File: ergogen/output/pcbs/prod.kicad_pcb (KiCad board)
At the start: 2 copper layers, 220.4 x 89.6 mm, 63 parts

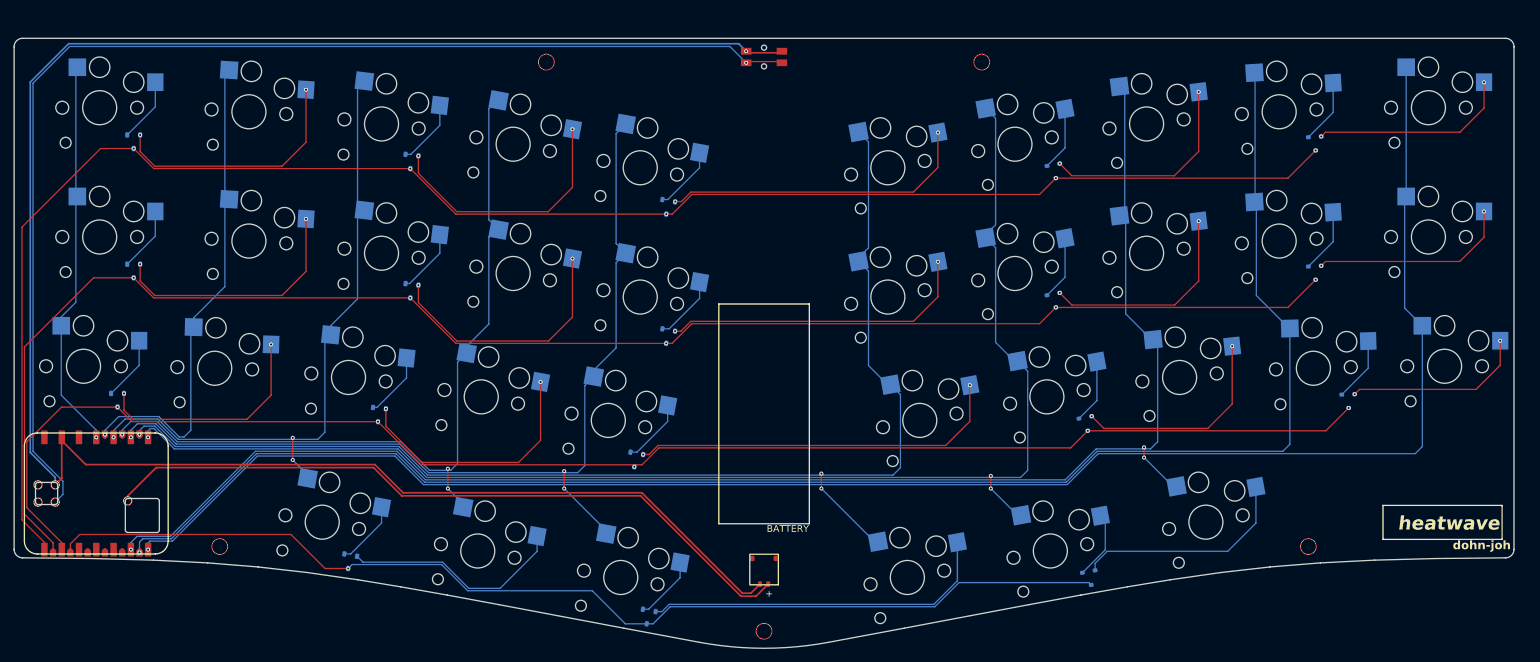
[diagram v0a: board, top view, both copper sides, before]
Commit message: release
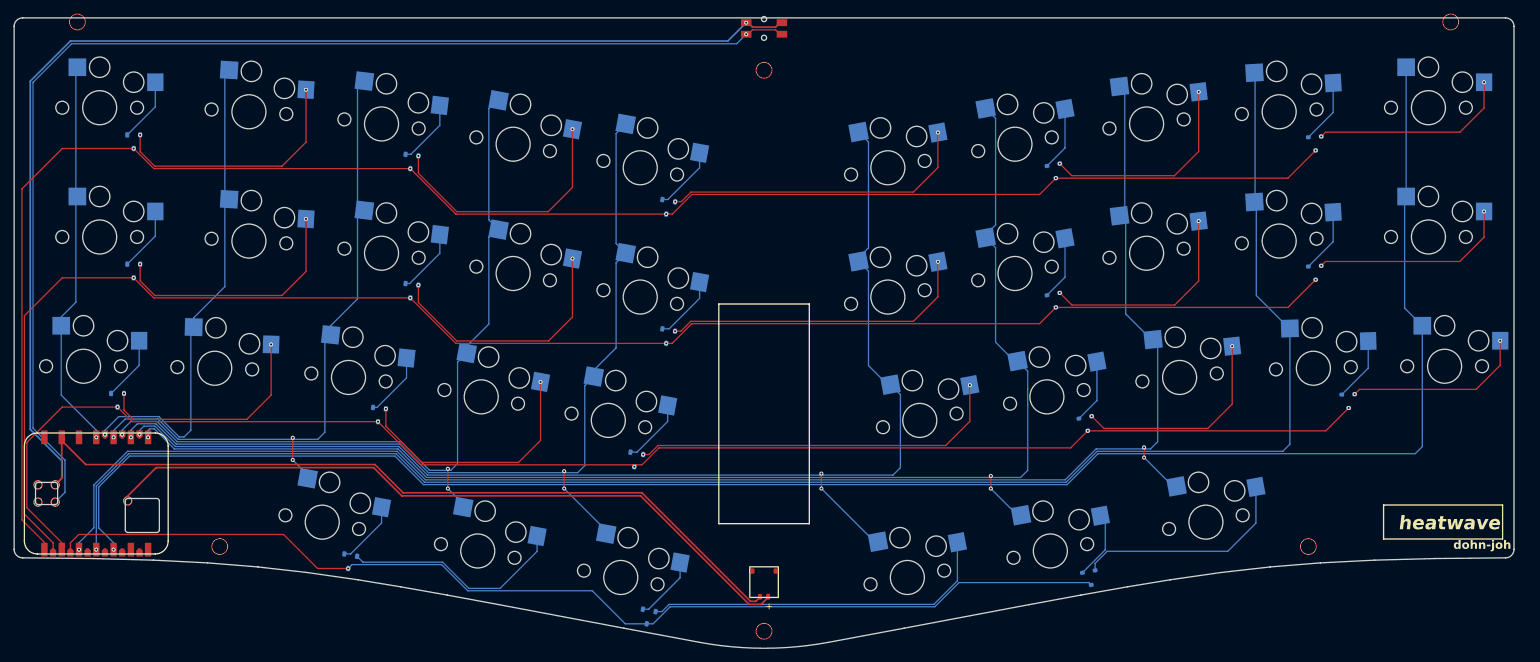
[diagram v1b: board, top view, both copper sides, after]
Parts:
- added H6: , mounting_hole, F.Cu at (177.6, 64.5)
- moved H3 196.7 mm to (198.6, -12.6)
- moved H4 81.0 mm to (17.6, 64.5)
- moved H5 81.0 mm to (97.6, 76.9)
- moved H1 69.2 mm to (-3.27, -12.6)
- moved H2 32.0 mm to (97.6, -5.50)
- moved XX1 4.20 mm to (97.6, -11.7)
- moved XX2 1.85 mm to (97.6, 70.0)
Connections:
- MCU1 pad 3: P0.28 -> C8
- MCU1 pad 4: P0.29 -> C9
- MCU1 pad 5: P0.04 -> C10
- MCU1 pad 6: C8 -> P0.05
- MCU1 pad 7: C10 -> P1.11
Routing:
- net C10: track 254.5 -> 267.5 mm
- net C8: track 225.1 -> 236.4 mm
- net C9: track 236.9 -> 247.7 mm
- net R1: track 251.6 -> 254.9 mm
- net R2: track 233.8 -> 236.5 mm
- net GND: track 294.5 -> 296.9 mm
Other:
- board size 220.4 x 89.6 mm -> 220.4 x 92.6 mm
- board text removed: "BATTERY"
